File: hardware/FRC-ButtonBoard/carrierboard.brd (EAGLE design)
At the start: 81 x 85.1 mm, 36 parts

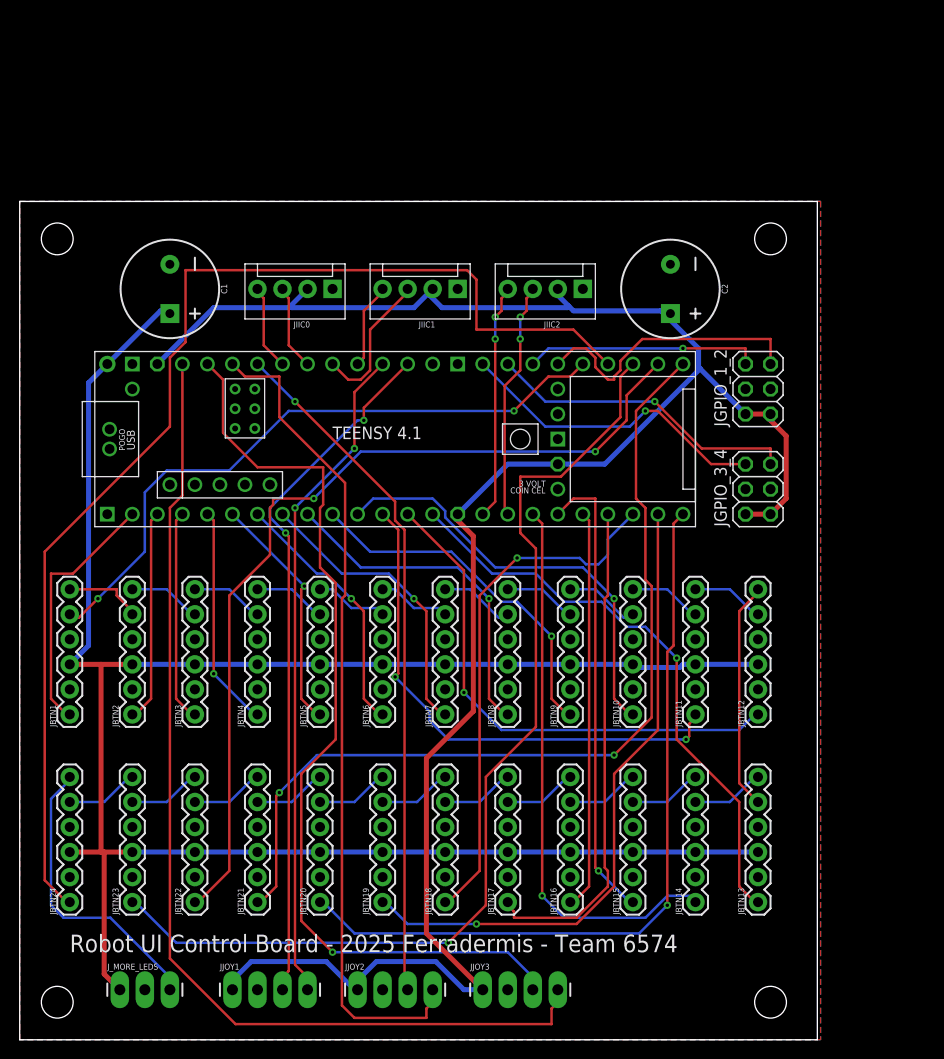
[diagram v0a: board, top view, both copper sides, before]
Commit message: commit to more buttons
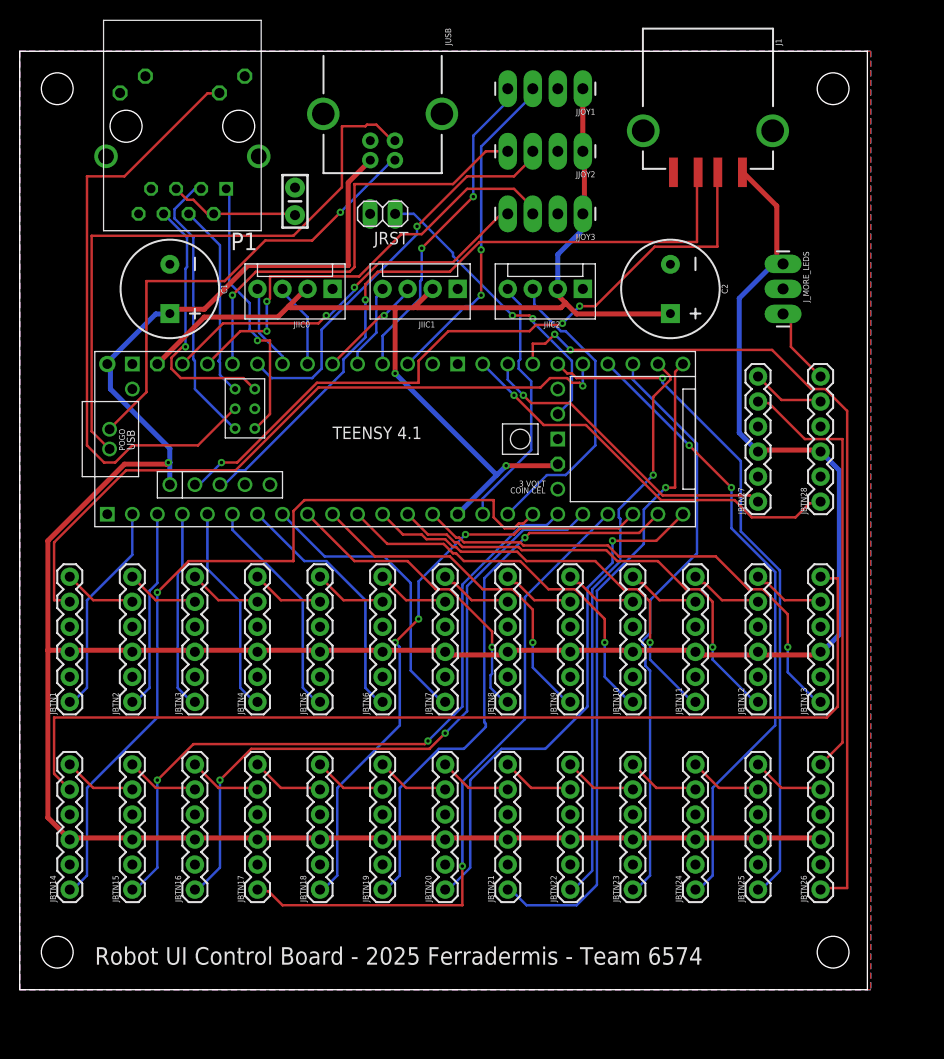
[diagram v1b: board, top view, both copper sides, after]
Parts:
- removed JGPIO_1_2, JGPIO_3_4: (no value), pinhead:2X03
- added C3: 0.1uF, SparkFun-Capacitors:CAP-PTH-SMALL-KIT
- added J1: USB_A_SMT_FEMALE, SparkFun-Connectors:USB-A-S-SILK-FEMALE
- added JBTN25, JBTN26, JBTN27, JBTN28: (no value), SparkFun-Connectors:1X06
- added JRST: (no value), pinhead:1X02
- added JUSB: USB_B_PTH, SparkFun-Connectors:USB-B-PTH
- added P1: J1B1211CCD, WIZnet:J1B1211CCD
- moved J_MORE_LEDS 99.8 mm to (74.9, 76.2), turned to 270 degrees
- moved JJOY1 98.1 mm to (54.6, 94.0), turned to 180 degrees
- moved JJOY2 88.1 mm to (54.6, 87.6), turned to 180 degrees
- moved JJOY3 79.4 mm to (54.6, 81.3), turned to 180 degrees
- moved JBTN14 63.5 mm to (2.54, 12.7)
- moved JBTN24 63.5 mm to (66.0, 12.7)
- moved JBTN15 50.8 mm to (8.89, 12.7)
- moved JBTN23 50.8 mm to (59.7, 12.7)
- moved JBTN16 38.1 mm to (15.2, 12.7)
- moved JBTN22 38.1 mm to (53.3, 12.7)
- moved JBTN17 25.4 mm to (21.6, 12.7)
- moved JBTN21 25.4 mm to (47.0, 12.7)
- moved JBTN13 21.3 mm to (78.7, 31.8)
- moved JBTN18 12.8 mm to (27.9, 12.7)
- moved JBTN20 12.8 mm to (40.6, 12.7)
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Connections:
- removed net GPIO1: JGPIO_1_2.5, U$1.38-A14/CS/IN1
- removed net GPIO2: JGPIO_1_2.6, U$1.39-A15/CS/OUT1A
- removed net GPIO3: JGPIO_3_4.5, U$1.40-A16/CS1
- removed net GPIO4: JGPIO_3_4.6, U$1.41-A17/MISO1
- new net B25_DIN: JBTN24.6, JBTN25.5
- new net B26_DIN: JBTN25.6, JBTN26.5
- new net B27_DIN: JBTN26.6, JBTN27.5
- new net B28_DIN: JBTN27.6, JBTN28.5
- new net BTN25: JBTN25.1, U$1.38-A14/CS/IN1
- new net BTN26: JBTN26.1, U$1.39-A15/CS/OUT1A
- new net BTN27: JBTN27.1, U$1.40-A16/CS1
- new net BTN28: JBTN28.1, U$1.41-A17/MISO1
- new net ETH_LED: P1.10, U$1.LED
- new net ETH_R+: P1.4, U$1.R+
- new net ETH_R-: P1.6, U$1.R-
- new net ETH_T+: P1.1, U$1.T+
- new net ETH_T-: P1.3, U$1.T-
- new net N$1: C3.2, P1.2, P1.5
- new net N$10: U$1.VUSB
- new net PROGRAM_RESET: JRST.1, U$1.PROGRAM
- new net USBH_D+: J1.D+, U$1.DP
- new net USBH_D-: J1.D-, U$1.DM
- new net USB_D+: JUSB.D+, U$1.D+
- new net USB_D-: JUSB.D-, U$1.D-
- net 3V3: no longer JGPIO_1_2.1, JGPIO_1_2.2, JGPIO_3_4.1, JGPIO_3_4.2
- net 5V: now also J1.VBUS, JBTN25.3, JBTN26.3, JBTN27.3, JBTN28.3, JUSB.VBUS, U$1.+5V
- net B_DOUT: now also JBTN28.6; no longer JBTN24.6
- net GND: now also C3.1, J1.GND, J1.SHLD1, J1.SHLD2, JBTN25.2, JBTN25.4, JBTN26.2, JBTN26.4, JBTN27.2, JBTN27.4, JBTN28.2, JBTN28.4, JRST.2, JUSB.GND, JUSB.SHLD1, JUSB.SHLD2, P1.13, P1.14, P1.8, P1.9, U$1.G; no longer JGPIO_1_2.3, JGPIO_1_2.4, JGPIO_3_4.3, JGPIO_3_4.4
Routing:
- net 5V: track 214.6 -> 322.7 mm, vias 0 -> 1
- net B14_DIN: track 7.40 -> 102.8 mm
- net 3V3: track 209.6 -> 117.4 mm, vias 0 -> 2
- net BTN26: track 0.00 -> 88.8 mm, vias 0 -> 2
- net USBH_D-: track 0.00 -> 71.9 mm, vias 0 -> 3
- net USBH_D+: track 0.00 -> 69.7 mm, vias 0 -> 1
- net BTN25: track 0.00 -> 69.2 mm, vias 0 -> 1
- net JOY_S2: track 106.1 -> 39.5 mm, vias 0 -> 2
- net ETH_LED: track 0.00 -> 62.3 mm
- net USB_D+: track 0.00 -> 62.1 mm
- net BTN24: track 121.1 -> 63.9 mm, vias 0 -> 2
- net JOY_S1: track 94.7 -> 44.9 mm, vias 1 -> 2
- net USB_D-: track 0.00 -> 47.0 mm, vias 0 -> 1
- net BTN23: track 104.0 -> 59.6 mm, vias 1 -> 0
- net B27_DIN: track 0.00 -> 44.1 mm
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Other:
- board size 81 x 85.1 mm -> 86 x 95.2 mm
